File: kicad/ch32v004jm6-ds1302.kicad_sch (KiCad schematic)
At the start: 10 parts, among them J2 Conn_01x03_Pin, SW1 SW_Push, U2 DS1302+, Y1 Crystal

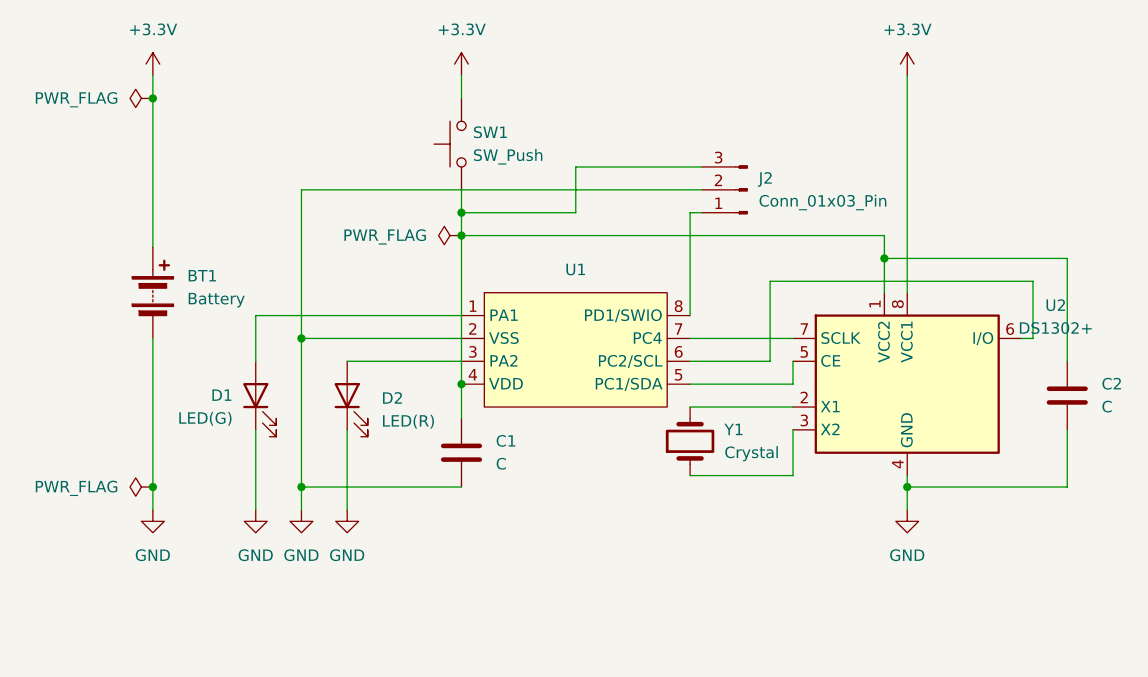
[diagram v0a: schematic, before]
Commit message: Update CAD data
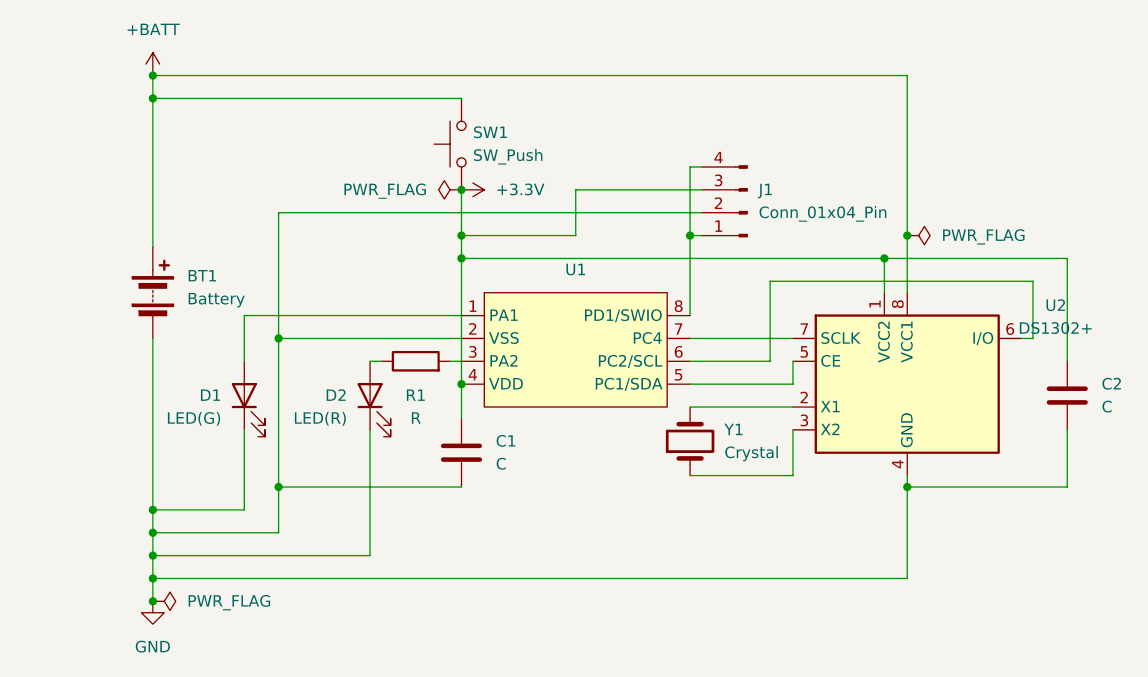
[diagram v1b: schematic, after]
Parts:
- removed J2: Conn_01x03_Pin, Connector_PinSocket_2.54mm:PinSocket_2x02_P2.54mm_Vertical, symbol Connector:Conn_01x03_Pin
- added J1: Conn_01x04_Pin, Connector_PinSocket_2.54mm:PinSocket_2x02_P2.54mm_Vertical, symbol Connector:Conn_01x04_Pin
- added R1: R, Resistor_SMD:R_0603_1608Metric, symbol Device:R
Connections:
- net +3.3V: now also C1.1, C2.1, SW1.1, U1.4 (VDD), U2.1 (VCC2), J1.3 (Pin_3); no longer BT1.1 (+), SW1.2, U2.8 (VCC1)
- net GND: now also J1.2 (Pin_2)
- net at U1.8 (PD1/SWIO): now also J1.1 (Pin_1), J1.4 (Pin_4)
- net at D2.2 (A): now also R1.1; no longer U1.3 (PA2)
- new net: R1.2, U1.3 (PA2)
- new net +BATT: BT1.1 (+), SW1.2, U2.8 (VCC1)
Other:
- moved on the sheet: D1, D2
